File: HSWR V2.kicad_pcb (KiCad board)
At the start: 4 copper layers, 152 x 139 mm, 161 parts, among them IC1 ADM3052, IC2 TPS65320C, IC4 INA240A1, IC5 INA240A1, P1 USB_B, P2 Interface, P3 IN+, P4 IN-, P5 MOTOR3, P6 MOTOR2, P7 MOTOR1, P8 SWD, Q1 ZXTC2045E6, Q10 ZXTC2045E6, Q11 IRFP4668PBF, Q12 IRFP4668PBF, Q2 ZXTC2045E6, Q3 IRFP4668PBF, Q4 IRFP4668PBF, Q5 ZXTC2045E6, Q6 ZXTC2045E6, Q7 IRFP4668PBF, Q8 IRFP4668PBF, Q9 ZXTC2045E6, U1 STM32F40X_LQFP64, U2 IR2110S, U3 IR2110S, U4 IR2110S, X1 8MHz 10ppm

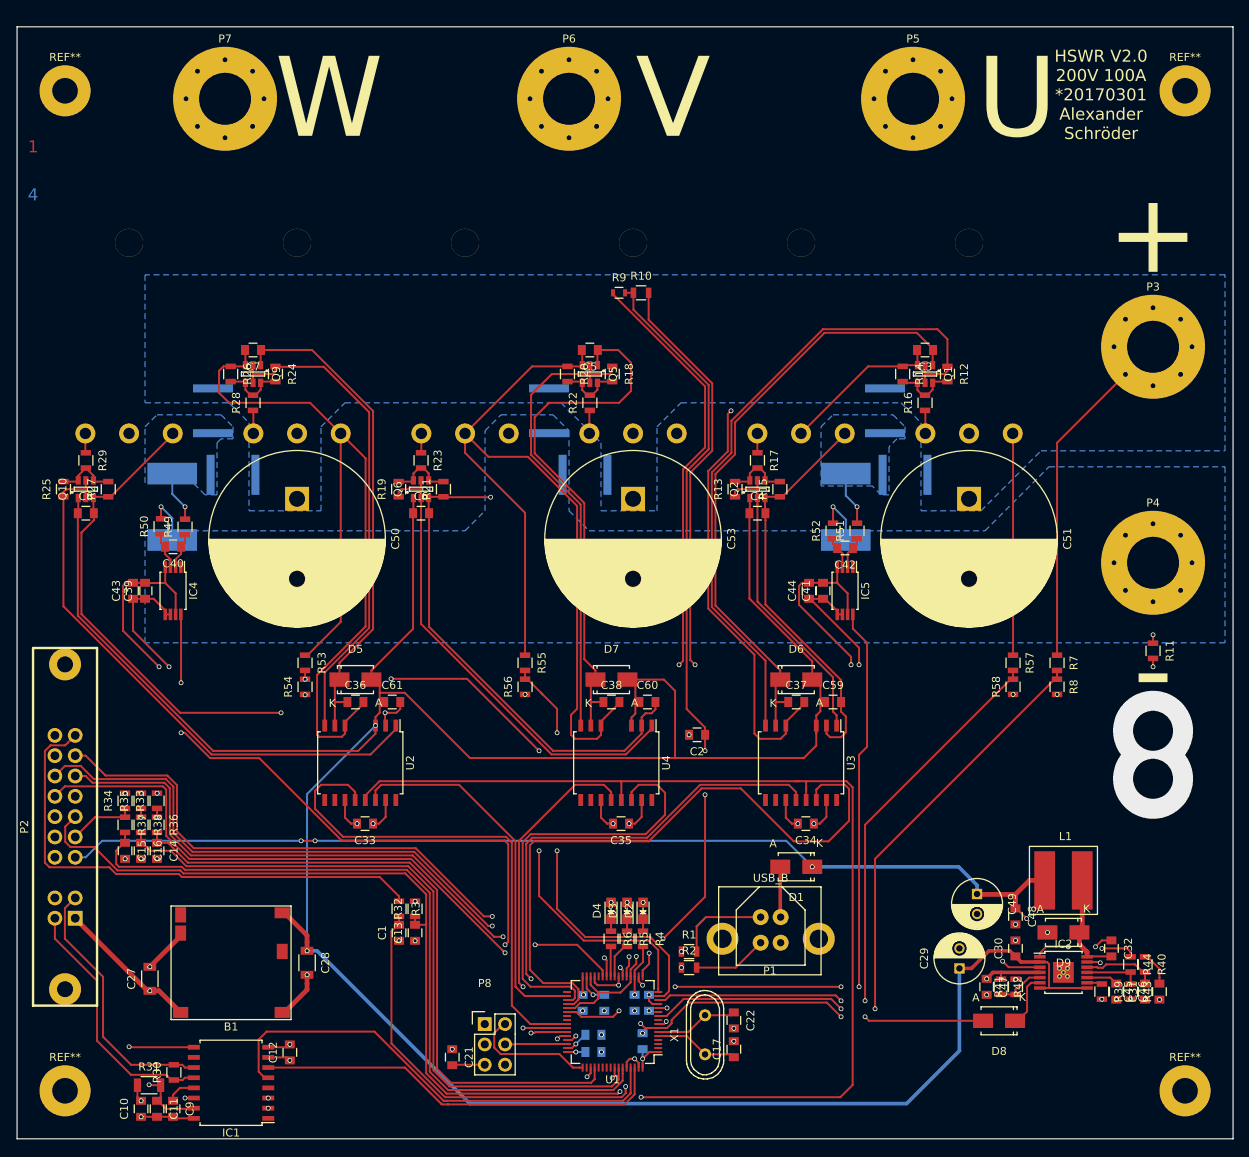
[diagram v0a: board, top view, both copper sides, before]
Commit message: - updated project to 5.0.0 - added ignore file
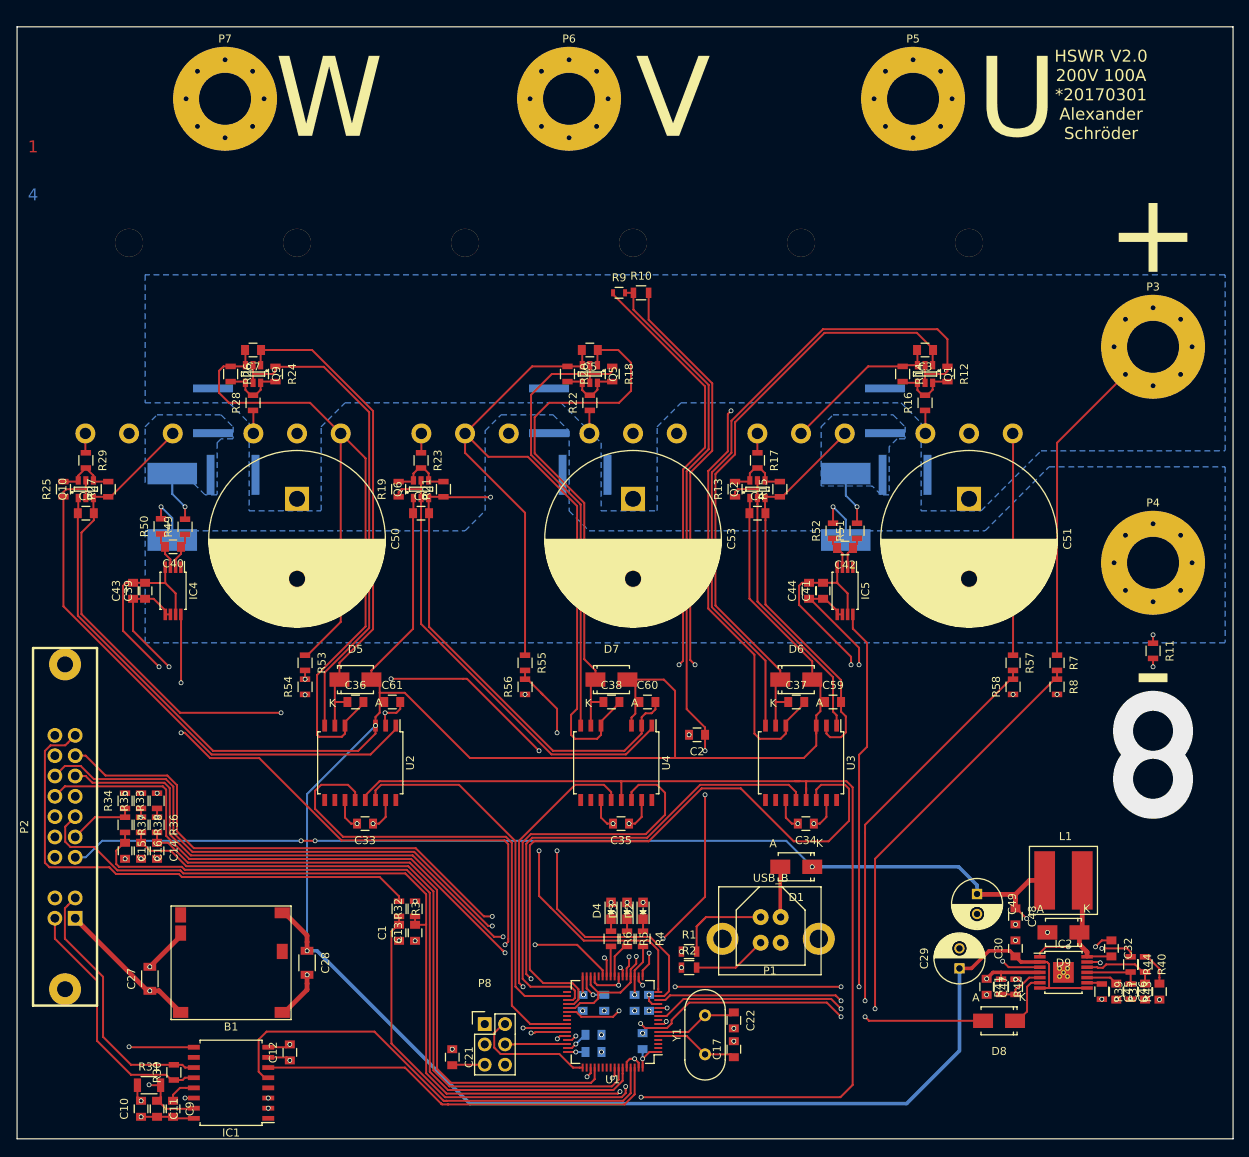
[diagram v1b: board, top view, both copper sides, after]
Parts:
- removed REF** (x4): MountingHole_3.2mm_M3_Pad, Mounting_Holes:MountingHole_3.2mm_M3_Pad
- removed X1: 8MHz 10ppm, Crystals:Crystal_HC49-U_Vertical
- added Y1: 8MHz, Crystals:Crystal_HC49-U_Vertical, F.Cu at (153.0, 152.4)
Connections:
- B1 pad 3: (no net) -> Net-(B1-Pad3)
- B1 pad 5: (no net) -> Net-(B1-Pad5)
- C12 pad 2: GND -> Net-(C12-Pad2)
- C9 pad 2: Earth -> Net-(C9-Pad2)
- IC1 pad 10: (no net) -> Net-(IC1-Pad10)
- IC1 pad 16: Earth -> Net-(C9-Pad2)
- IC1 pad 2: GND -> Net-(C12-Pad2)
- IC1 pad 3: GND -> Net-(IC1-Pad3)
- IC1 pad 4: (no net) -> /CAN bus transceiver/V+Sense
- P8 pad 6: (no net) -> Net-(P8-Pad6)
- U1 pad 11: (no net) -> Net-(U1-Pad11)
- U1 pad 2: (no net) -> Net-(U1-Pad2)
- U1 pad 28: (no net) -> Net-(U1-Pad28)
- U1 pad 3: (no net) -> Net-(U1-Pad3)
- U1 pad 33: (no net) -> /MCU/DC_CAL
- U1 pad 39: (no net) -> Net-(U1-Pad39)
- U1 pad 4: (no net) -> Net-(U1-Pad4)
- U1 pad 40: (no net) -> Net-(U1-Pad40)
- U1 pad 50: (no net) -> Net-(U1-Pad50)
- U1 pad 53: (no net) -> /MCU/FAULT
- U1 pad 54: (no net) -> Net-(U1-Pad54)
- U1 pad 55: (no net) -> Net-(U1-Pad55)
- U1 pad 56: (no net) -> Net-(U1-Pad56)
- U1 pad 9: (no net) -> Net-(U1-Pad9)
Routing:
- net Net-(IC1-Pad3): vias 0 -> 1
- net Net-(C12-Pad2): vias 0 -> 1
- net GND: vias 50 -> 48
